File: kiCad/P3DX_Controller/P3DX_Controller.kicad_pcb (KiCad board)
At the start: 2 copper layers, 125 x 80 mm, 25 parts, among them J1 Conn_01x10_Pin, J2 Conn_01x26_Pin, J3 Conn_01x10_Pin, J4 Conn_01x16_Pin, J5 Conn_01x03_Pin, J6 Conn_01x05_Pin, U1 TXS0108EPW, U3 ESP32-DevKitC

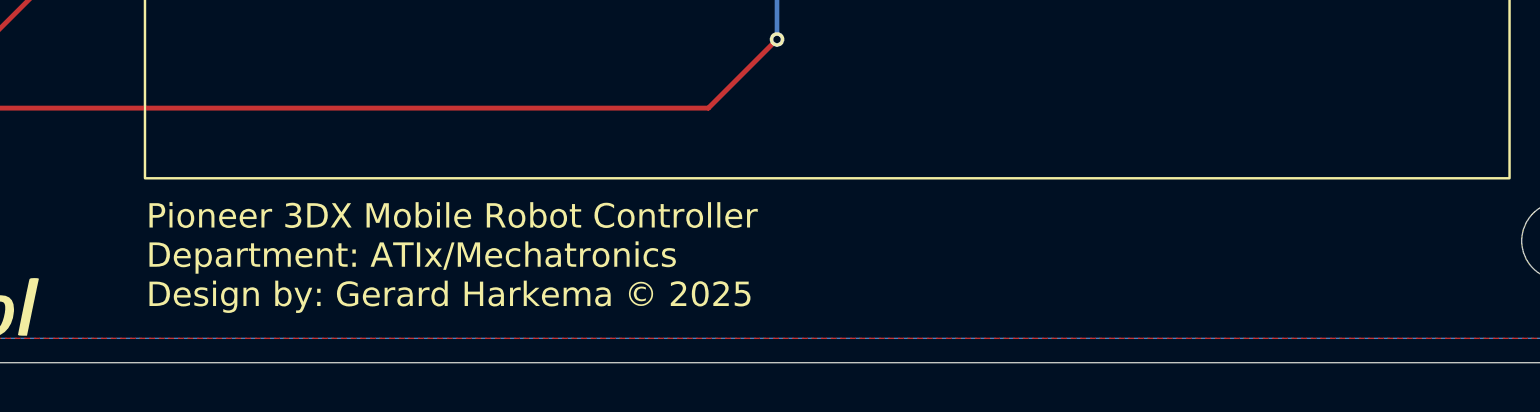
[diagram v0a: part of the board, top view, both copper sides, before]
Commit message: 20251201
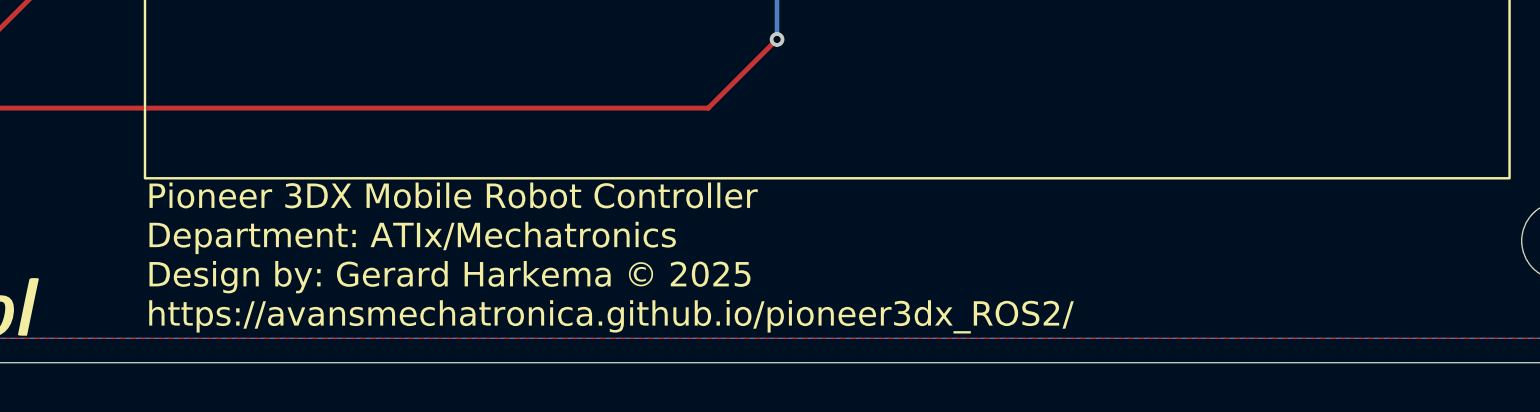
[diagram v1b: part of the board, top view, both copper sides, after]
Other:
- board text added: "Pioneer 3DX Mobile Robot Controller Department: ATIx/Mechatronics Design by: Gerard Harkema © 2025 https://avansmechatronica.github.io/pioneer3dx_ROS2/"
- board text removed: "Pioneer 3DX Mobile Robot Controller Department: ATIx/Mechatronics Design by: Gerard Harkema © 2025"
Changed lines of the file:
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@@
 		)
 	)
-	(gr_text "Pioneer 3DX Mobile Robot Controller\nDepartment: ATIx/Mechatronics\nDesign by: Gerard Harkema © 2025\n"
+	(gr_text "Pioneer 3DX Mobile Robot Controller\nDepartment: ATIx/Mechatronics\nDesign by: Gerard Harkema © 2025\nhttps://avansmechatronica.github.io/pioneer3dx_ROS2/"
 		(locked yes)
 		(at 111.95 125.6 0)
